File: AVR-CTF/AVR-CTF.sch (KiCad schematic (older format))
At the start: 0 parts

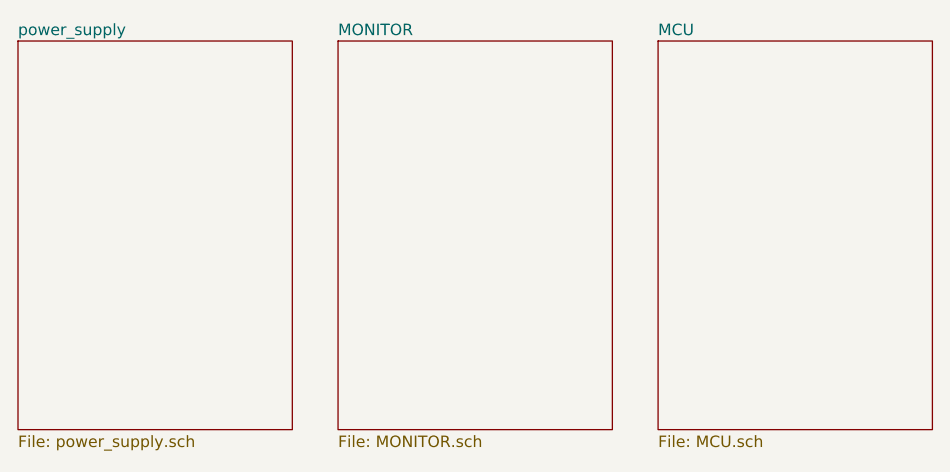
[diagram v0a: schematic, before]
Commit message: Esquematico para revision
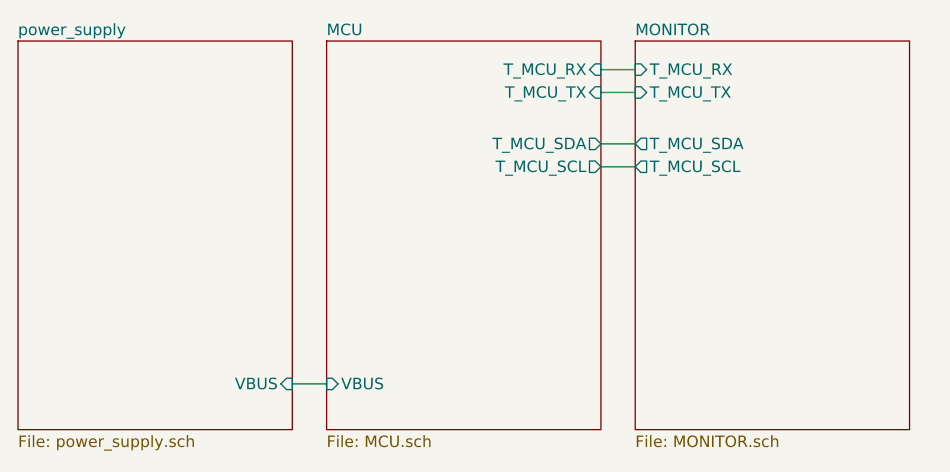
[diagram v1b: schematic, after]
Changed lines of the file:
@@
 F0 "power_supply" 50
 F1 "power_supply.sch" 50
+F2 "VBUS" I R 3000 3500 50
 $EndSheet
 $Sheet
-S 3200 2000 1200 1700
+S 4500 2000 1200 1700
 U 621FB334
 F0 "MONITOR" 50
 F1 "MONITOR.sch" 50
+F2 "T_MCU_RX" I L 4500 2125 50
+F3 "T_MCU_TX" I L 4500 2225 50
+F4 "T_MCU_SDA" O L 4500 2450 50
+F5 "T_MCU_SCL" O L 4500 2550 50
 $EndSheet
 $Sheet
-S 4600 2000 1200 1700
+S 3150 2000 1200 1700
 U 6220499D
 F0 "MCU" 50
 F1 "MCU.sch" 50
+F2 "T_MCU_RX" I R 4350 2125 50
+F3 "T_MCU_TX" I R 4350 2225 50
+F4 "T_MCU_SDA" O R 4350 2450 50
+F5 "T_MCU_SCL" O R 4350 2550 50
+F6 "VBUS" I L 3150 3500 50
 $EndSheet
+Wire Wire Line
+	4350 2125 4500 2125
+Wire Wire Line
+	4350 2225 4500 2225
+Wire Wire Line
+	4350 2450 4500 2450
+Wire Wire Line
+	4350 2550 4500 2550
+Wire Wire Line
+	3000 3500 3150 3500
 $EndSCHEMATC
